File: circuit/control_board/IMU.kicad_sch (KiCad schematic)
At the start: 24 parts, among them U3 ADIS16470AMLZ, U4 B0505S-1WR3, U5 HX9193, U6 π131M31, U7 π131M31

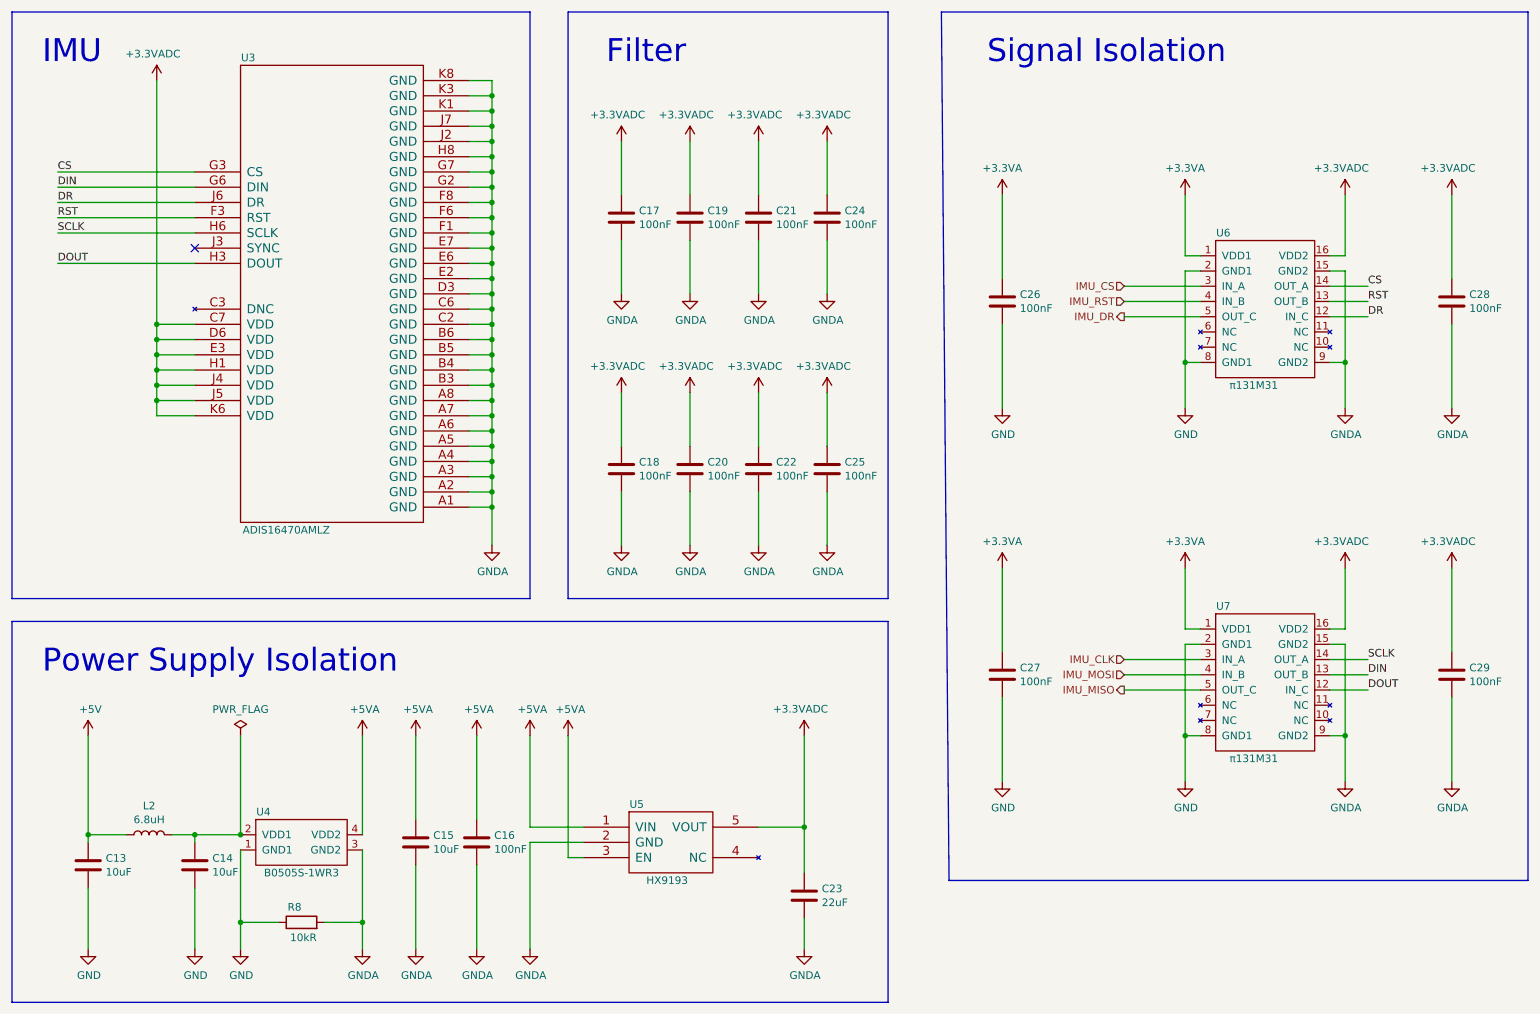
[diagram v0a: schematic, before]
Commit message: Modified the circuitry of the main control board to add a microcontroller for reading information from the magnetometer and IMU. Modified the SPI connection port of the Process MCU.
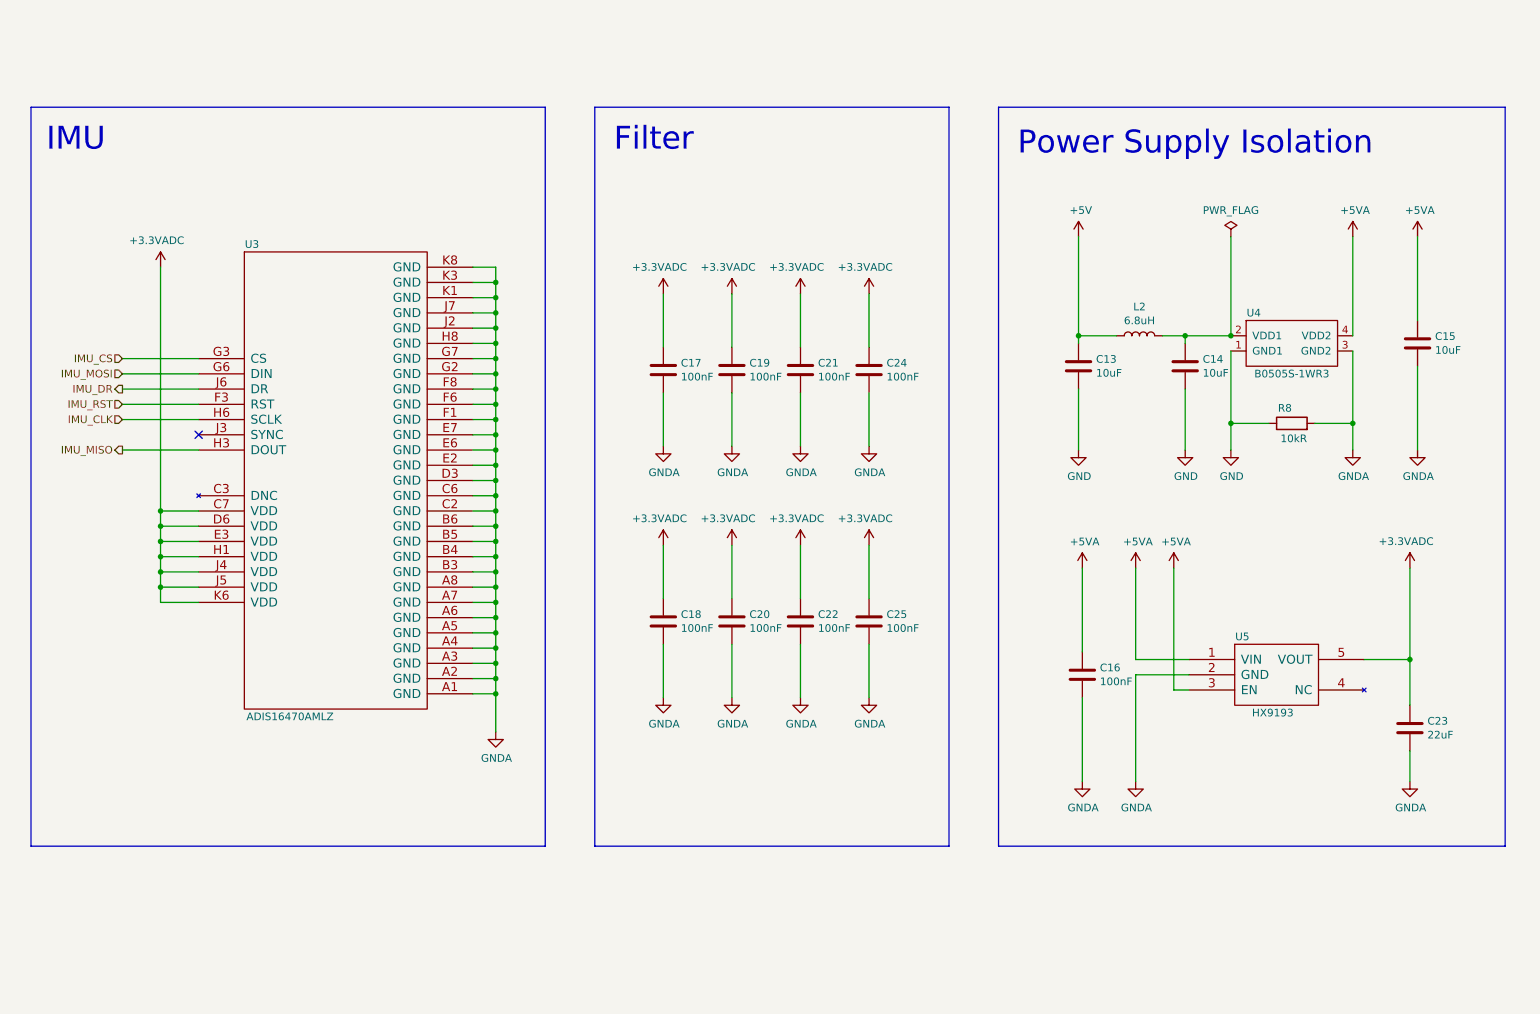
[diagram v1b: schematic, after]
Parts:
- removed C26, C27, C28, C29: 100nF, Capacitor_SMD:C_0603_1608Metric, symbol Device:C
- removed U6, U7: π131M31, Package_SO:SOIC-16_3.9x9.9mm_P1.27mm, symbol MM32_Periph:π131M31
- C13, C14, C15, C16, C17, C18, C19, C20, C21, C22, C23, C24, C25: footprint Capacitor_SMD:C_0603_1608Metric -> ControlBoard:C_0603_1608Metric
- L2: footprint Inductor_SMD:L_Abracon_ASPI-0630LR -> ControlBoard:L_Abracon_ASPI-0630LR
- R8: footprint Resistor_SMD:R_0603_1608Metric -> ControlBoard:R_0603_1608Metric
- U3: footprint MM32_Library:ADIS16470AMLZ -> ControlBoard:ADIS16470AMLZ
- U4: footprint MM32_Library:SIP-4_B0505S_1WR3 -> ControlBoard:SIP-4_B0505S_1WR3
- U5: footprint Package_TO_SOT_SMD:SOT-23-5 -> ControlBoard:SOT-23-5
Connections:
- net CS is gone; now on net IMU_CS: U3.G3 (CS)
- net DIN is gone; now on net IMU_MOSI: U3.G6 (DIN)
- net DOUT is gone; now on net IMU_MISO: U3.H3 (DOUT)
- net DR is gone; now on net IMU_DR: U3.J6 (DR)
- net RST is gone; now on net IMU_RST: U3.F3 (RST)
- net SCLK is gone; now on net IMU_CLK: U3.H6 (SCLK)
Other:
- note removed: "Signal Isolation"
- moved on the sheet: C13, C14, C15, C16, C17, C18, C19, C20, C21, C22, C23, C24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
